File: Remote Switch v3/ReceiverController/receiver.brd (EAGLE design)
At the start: 50 x 42 mm, 40 parts, among them IC1 LNK304, IC2 MCP1703CB, IC3 STM8L101F2, J1 POWER_CONN_4, T1 BT136

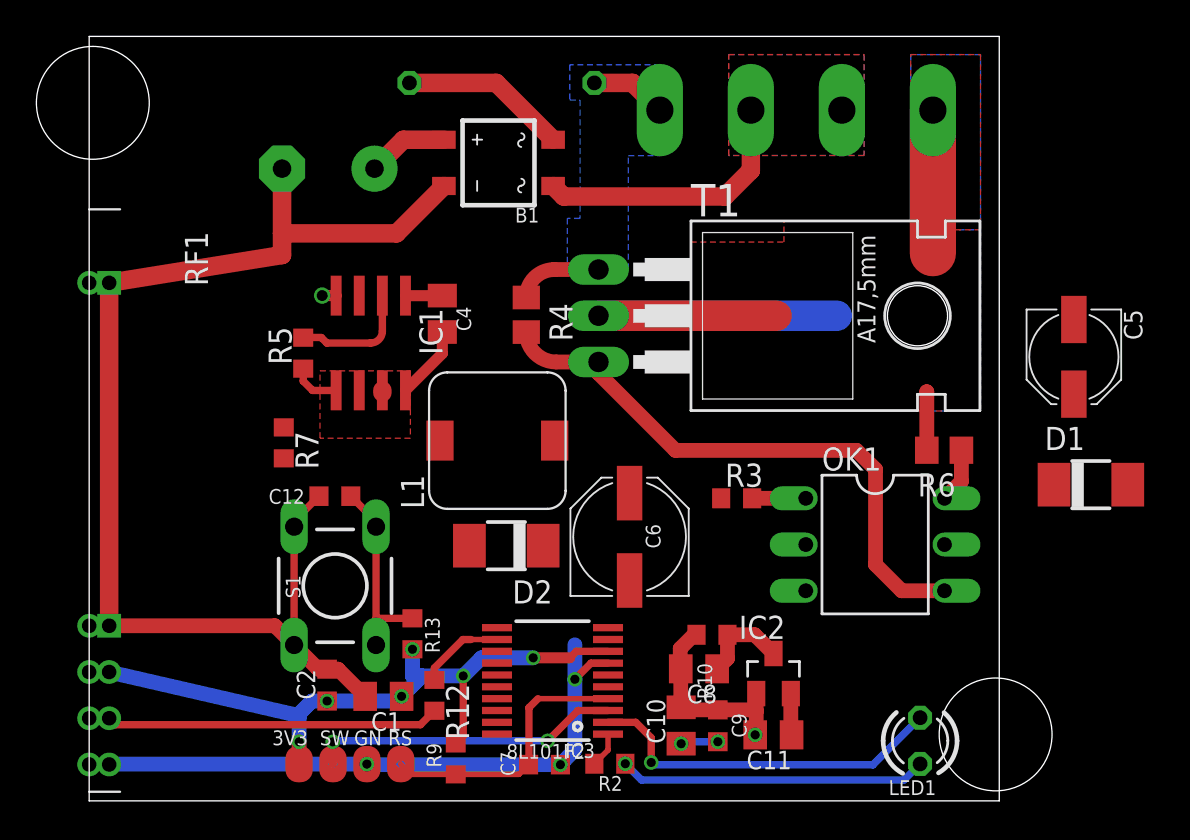
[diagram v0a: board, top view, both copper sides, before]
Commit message: PCB work
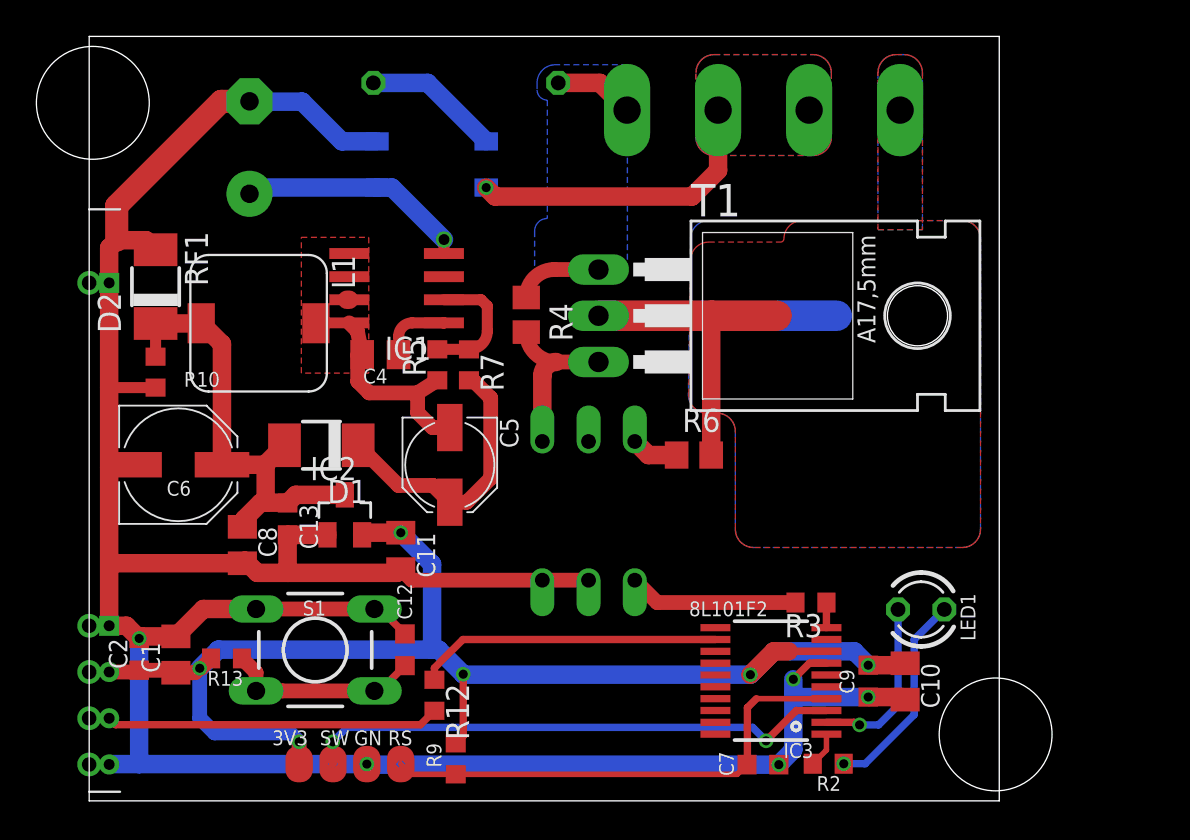
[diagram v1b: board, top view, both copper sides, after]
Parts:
- added C13: 100n, resistor:C0603K
- moved D1 42.3 mm to (13.8, 19.5), turned to 180 degrees
- moved C5 34.8 mm to (20.8, 18.5)
- moved R10 33.8 mm to (4.64, 23.6), turned to 90 degrees
- moved C8 26.0 mm to (9.42, 14.1), turned to 270 degrees
- moved IC2 25.1 mm to (15.0, 15.7)
- moved C6 25.1 mm to (5.89, 18.5), turned to 0 degrees
- moved D2 24.0 mm to (4.65, 28.3), turned to 90 degrees
- moved C11 22.8 mm to (18.1, 13.7), turned to 270 degrees
- moved OK1 15.9 mm to (28.4, 15.9), flipped to the bottom, turned to 0 degrees
- moved L1 14.6 mm to (10.3, 26.2), turned to 270 degrees
- moved R6 13.7 mm to (34.2, 19.0), turned to 0 degrees
- moved C10 12.5 mm to (45.8, 6.56), turned to 270 degrees
- moved C7 12.0 mm to (38.0, 1.99)
- moved IC3 12.0 mm to (38.5, 7.24)
- moved R2 12.0 mm to (41.6, 2.04)
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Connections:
- removed net N$19: B1.AC1, R1.1
- new net N$10: B1.AC2, R1.1
- net +5V: now also C13.1
- net GND: now also C13.2
- net N: now also B1.AC1; no longer B1.AC2
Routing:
- net GND: track 112.5 -> 153.6 mm, vias 4 -> 5
- net +3V3: track 42.1 -> 74.6 mm, vias 8 -> 6
- net N$8: track 32.3 -> 9.38 mm
- net +5V: track 5.06 -> 25.3 mm
- net N$3: track 0.00 -> 15.1 mm
- net SWIM: track 17.1 -> 29.7 mm
- net RST: track 15.3 -> 27.3 mm
- net N$9: track 4.74 -> 16.7 mm
- net LED_TX_ERR2: track 20.0 -> 9.71 mm
- net LOAD: track 40.1 -> 30.5 mm
- net N$19: track 9.19 -> 0.00 mm
- net N$1: track 5.24 -> 12.8 mm
- net N$10: track 0.00 -> 7.53 mm
- net N$11: track 2.95 -> 9.34 mm
- net N$2: track 16.9 -> 11.5 mm
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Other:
- board text added: "MOC3063"
